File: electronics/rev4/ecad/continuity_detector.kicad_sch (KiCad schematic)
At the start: 14 parts, among them U8 LMV761MF, U9 INA326

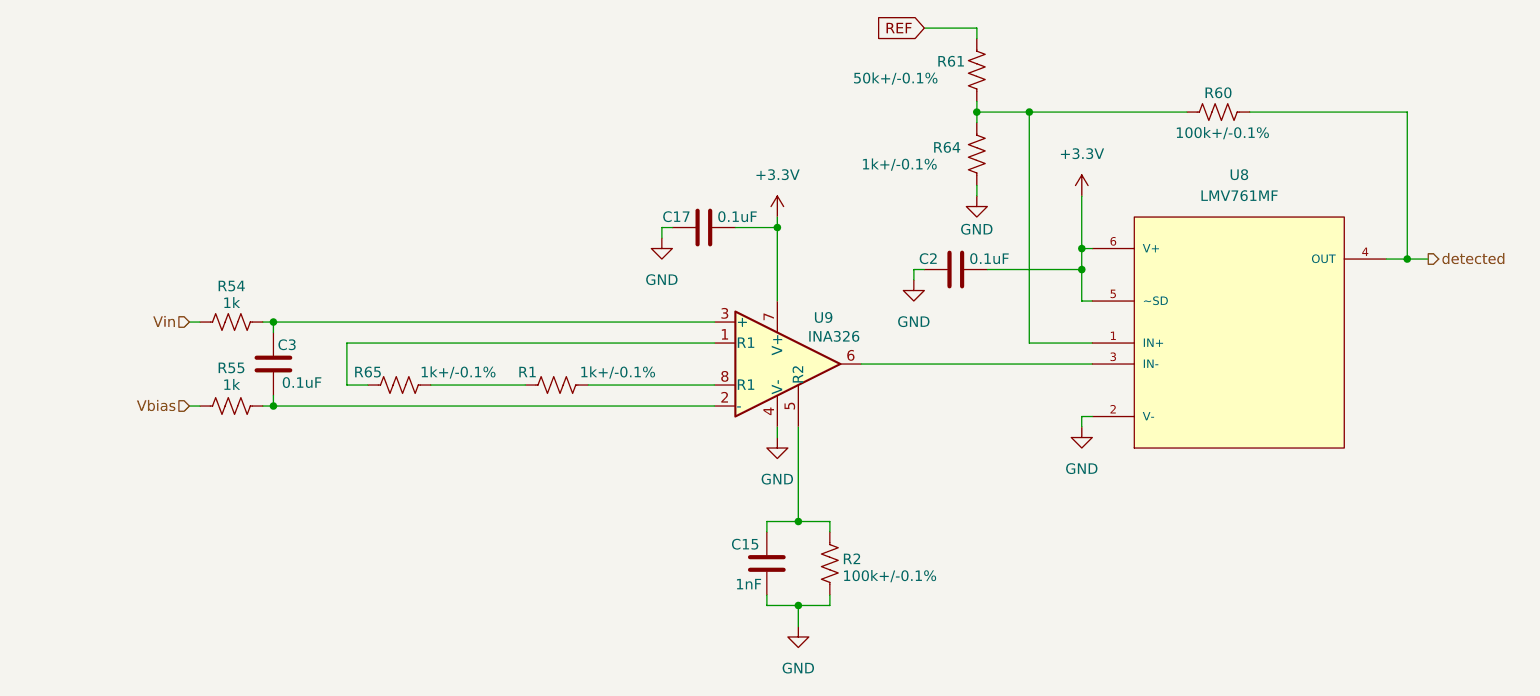
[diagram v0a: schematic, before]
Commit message: stuff
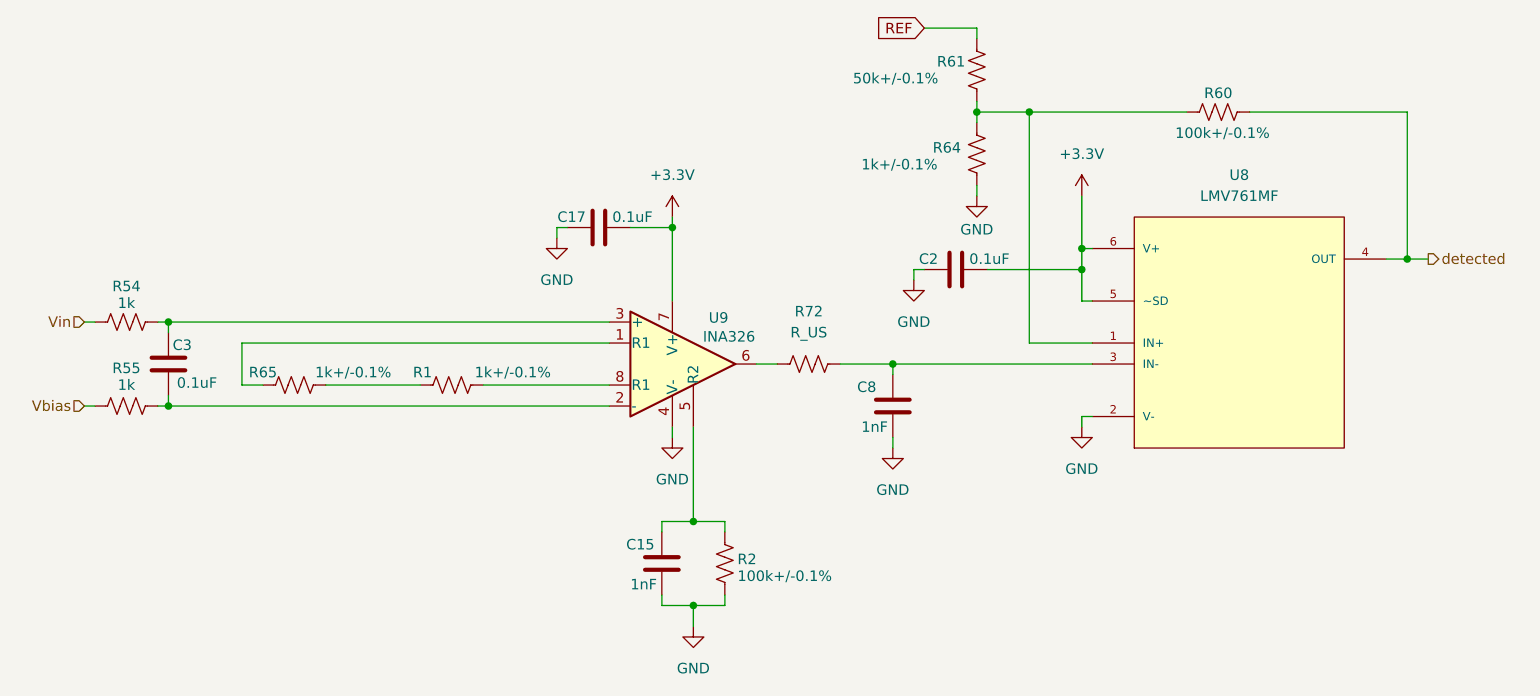
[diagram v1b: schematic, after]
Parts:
- added C8: 1nF, Capacitor_SMD:C_0805_2012Metric, symbol Device:C
- added R72: R_US, symbol Device:R_US
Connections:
- net GND: now also C8.2
- net at U9.6: now also R72.1; no longer U8.3 (IN-)
- new net: C8.1, R72.2, U8.3 (IN-)
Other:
- moved on the sheet: C15, C17, C3, R1, R2, R54, R55, R65, U9
